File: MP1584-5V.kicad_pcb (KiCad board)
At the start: 2 copper layers, 24.4 x 28 mm, 16 parts, among them J1 Conn_01x02, J2 Conn_01x02

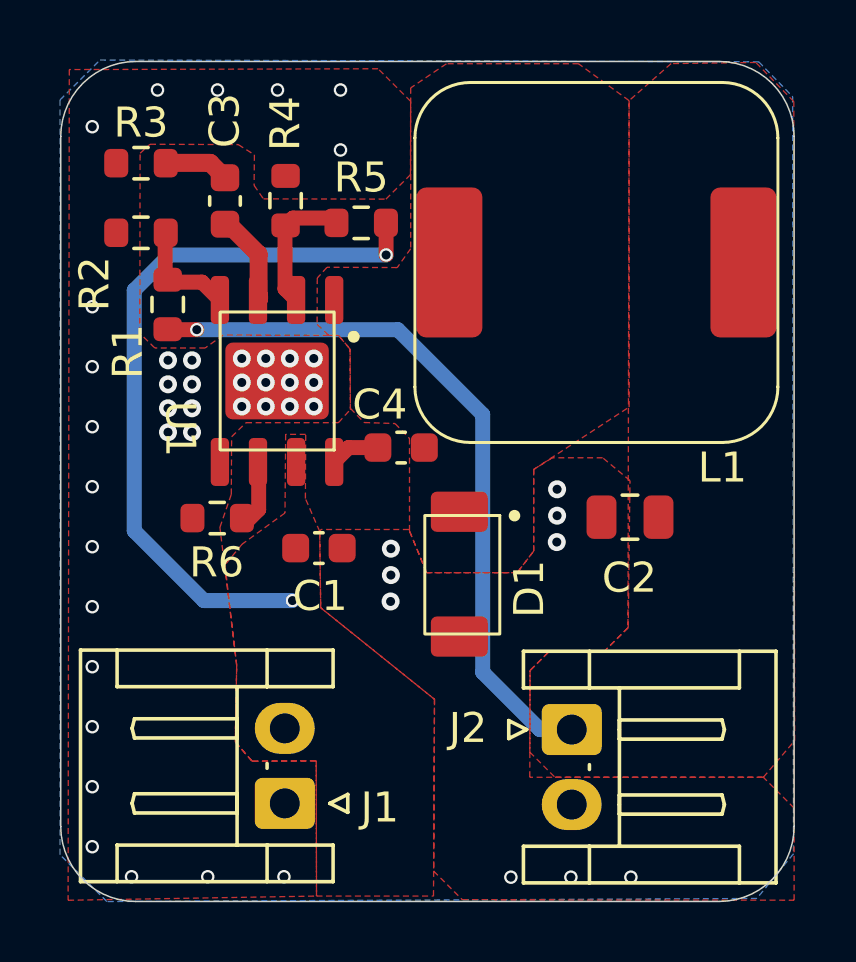
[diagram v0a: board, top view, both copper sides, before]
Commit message: amélioration finale + modification des photos du README
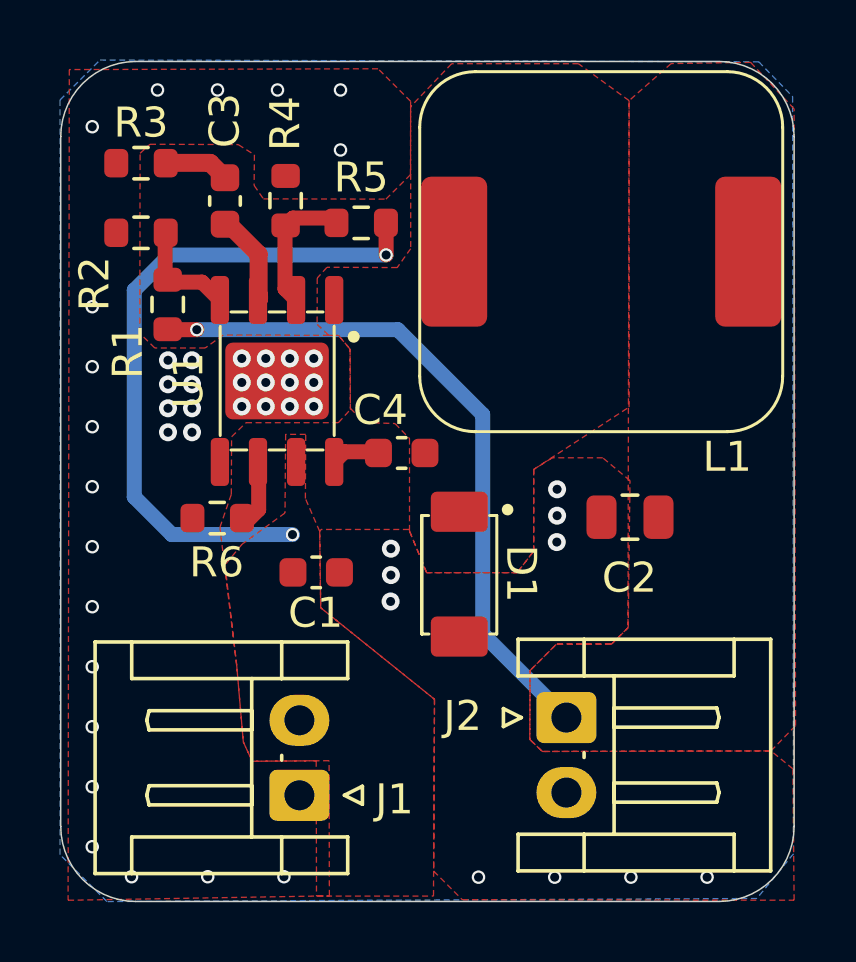
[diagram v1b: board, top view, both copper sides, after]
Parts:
- moved C1 0.81 mm to (162.0, 98.0)
- moved G*** 0.73 mm to (169.1, 86.7)
- moved J1 0.56 mm to (161.4, 105.5)
- moved J2 0.44 mm to (170.3, 102.9)
- moved L1 0.39 mm to (166.6, 87.3)
- moved C4 0.18 mm to (164.8, 94.0)
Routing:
- net /VIN: track 24.2 -> 22.6 mm
- net /Vout: track 24.0 -> 22.9 mm
- net GND: vias 48 -> 49
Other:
- board text added: "ARES ENSEA"
- board text added: "Buck-StepDown-28V-5V"
- board text added: "CAPODAGLI Janus"
- board text removed: "ARES ENSEA CAPODAGLI Janus"
